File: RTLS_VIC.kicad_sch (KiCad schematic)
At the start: 32 parts, among them J8 Conn_01x02_Pin, SW1 TS-1187A-B-A-B, U2 TPS63900DSKR, U9 STM32F411RET6, X1 XL2EL89COI-111YLC-26M

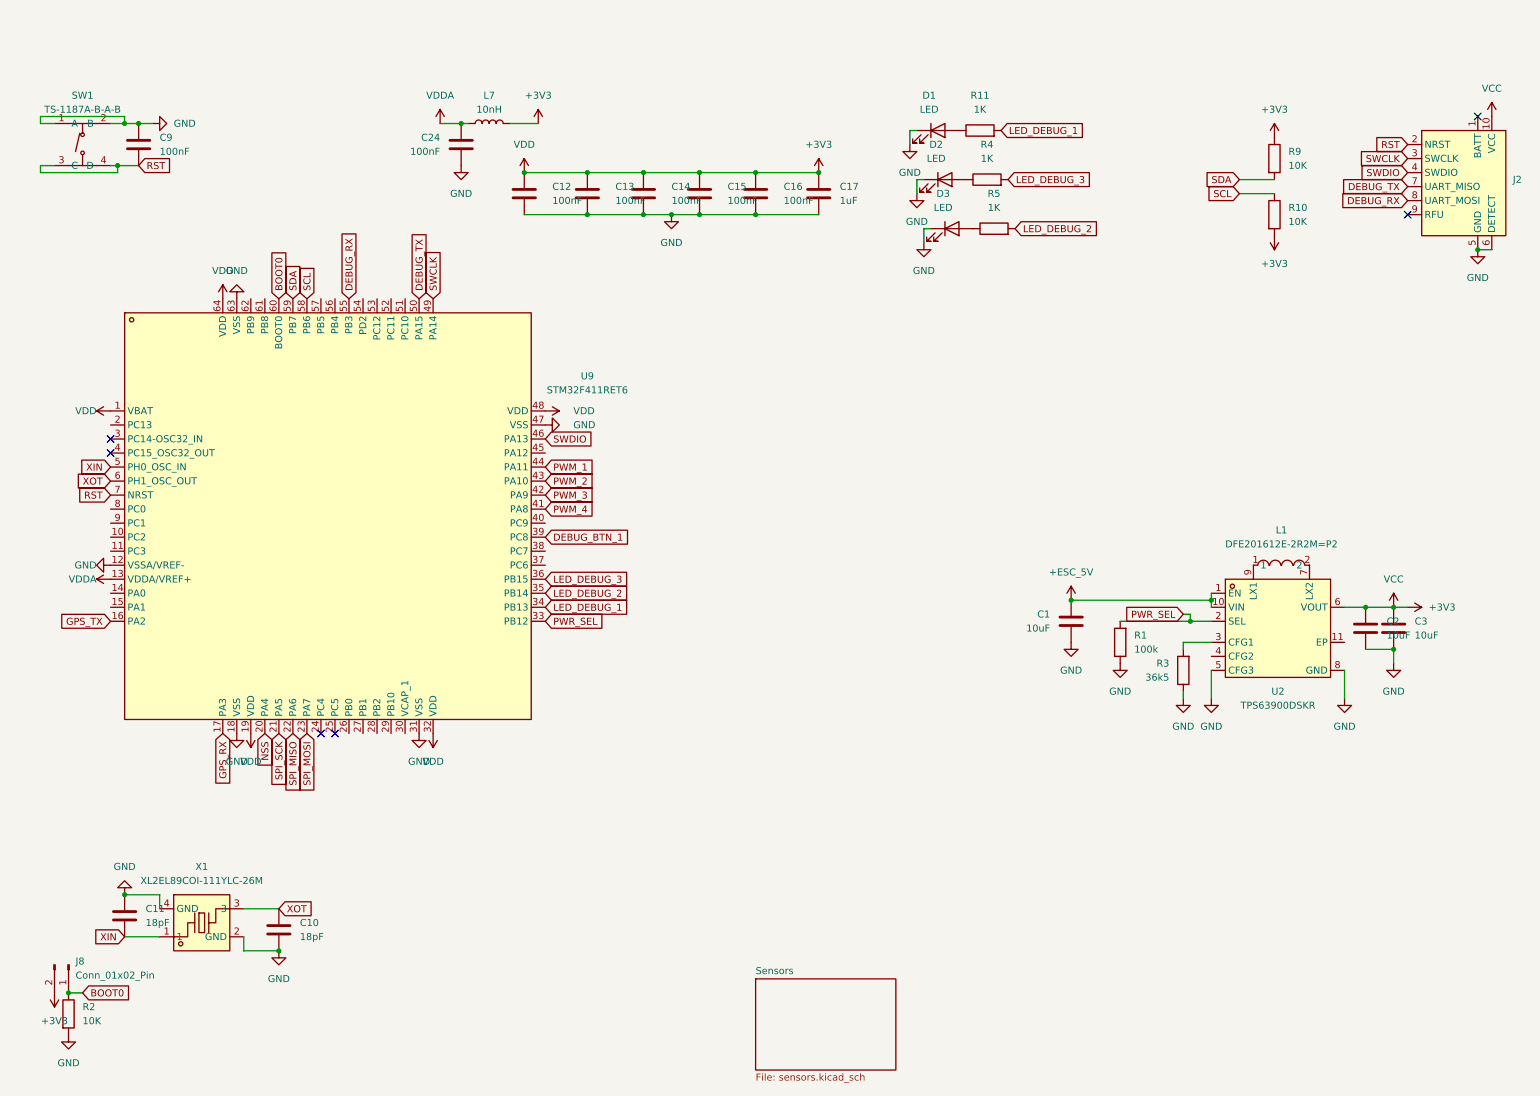
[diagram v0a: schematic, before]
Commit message: nearly there
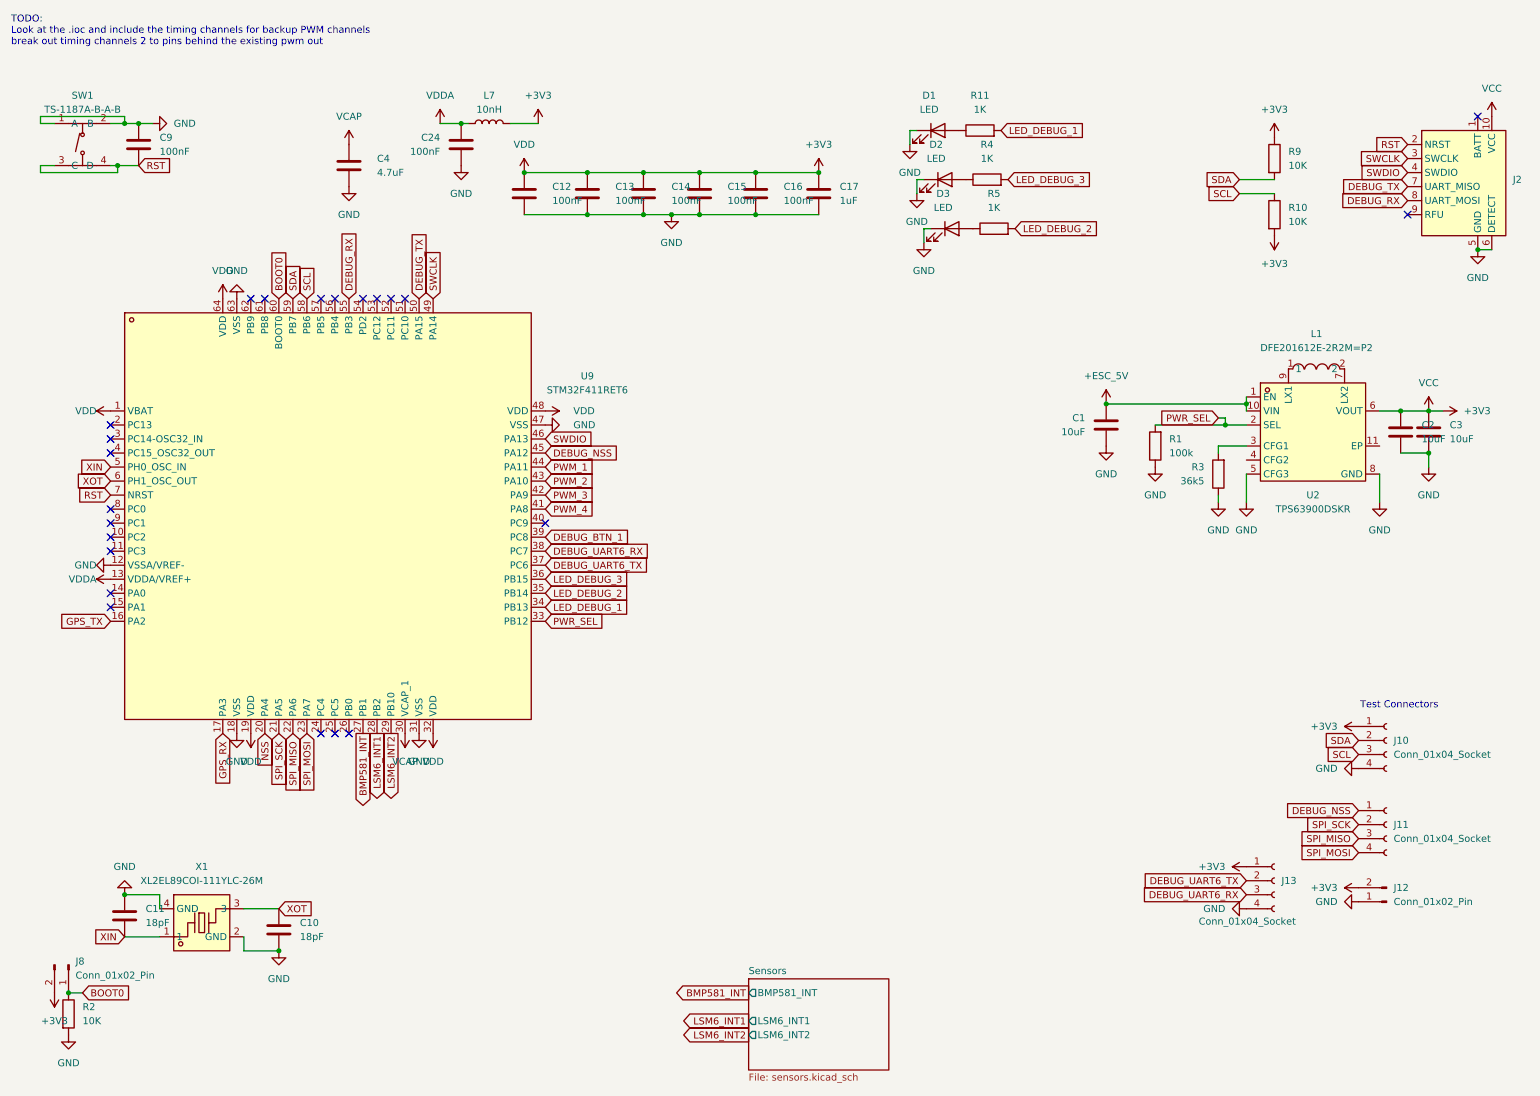
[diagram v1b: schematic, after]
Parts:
- added C4: 4.7uF, Capacitor_SMD:C_0402_1005Metric, symbol Device:C
- added J10, J11, J13: Conn_01x04_Socket, Connector_PinSocket_2.54mm:PinSocket_1x04_P2.54mm_Vertical, symbol Connector:Conn_01x04_Socket
- added J12: Conn_01x02_Pin, Connector_PinHeader_2.54mm:PinHeader_1x02_P2.54mm_Vertical, symbol Connector:Conn_01x02_Pin
- J8: now left out of the parts list
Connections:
- net +3V3: now also J10.1 (Pin_1), J12.2 (Pin_2), J13.1 (Pin_1)
- net GND: now also C4.2, J10.4 (Pin_4), J12.1 (Pin_1), J13.4 (Pin_4)
- net SCL: now also J10.3 (Pin_3)
- net SDA: now also J10.2 (Pin_2)
- net SPI_MISO: now also J11.3 (Pin_3)
- net SPI_MOSI: now also J11.4 (Pin_4)
- net SPI_SCK: now also J11.2 (Pin_2)
- net BMP581_INT: now reaches U9.27 (PB1)
- net LSM6_INT1: now reaches U9.28 (PB2)
- net LSM6_INT2: now reaches U9.29 (PB10)
- net VCAP: now reaches U9.30 (VCAP_1)
- net VCAP: now also C4.1
- net DEBUG_UART6_TX: now reaches U9.37 (PC6)
- net DEBUG_UART6_TX: now also J13.2 (Pin_2)
- net DEBUG_UART6_RX: now reaches U9.38 (PC7)
- net DEBUG_UART6_RX: now also J13.3 (Pin_3)
- net DEBUG_NSS: now reaches U9.45 (PA12)
- net DEBUG_NSS: now also J11.1 (Pin_1)
- no-connect marks 6 -> 23
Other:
- sheet Sensors ports: added BMP581_INT, LSM6_INT1, LSM6_INT2; removed none
- note added: "TODO: Look at the .ioc and include the timing channels for backup PWM channels break out timing channels 2 to pins behind the existing pwm out"
- note added: "Test Connectors"
- moved on the sheet: C1, C2, C3, L1, R1, R3, U2

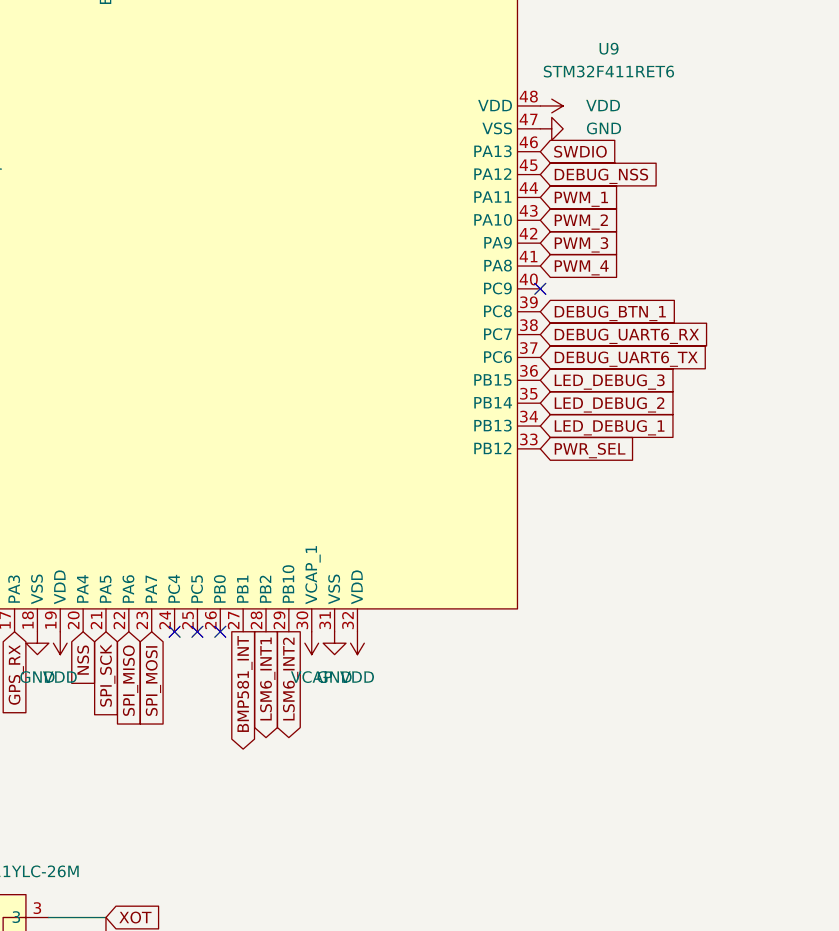
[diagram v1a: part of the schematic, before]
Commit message: preparing for prod
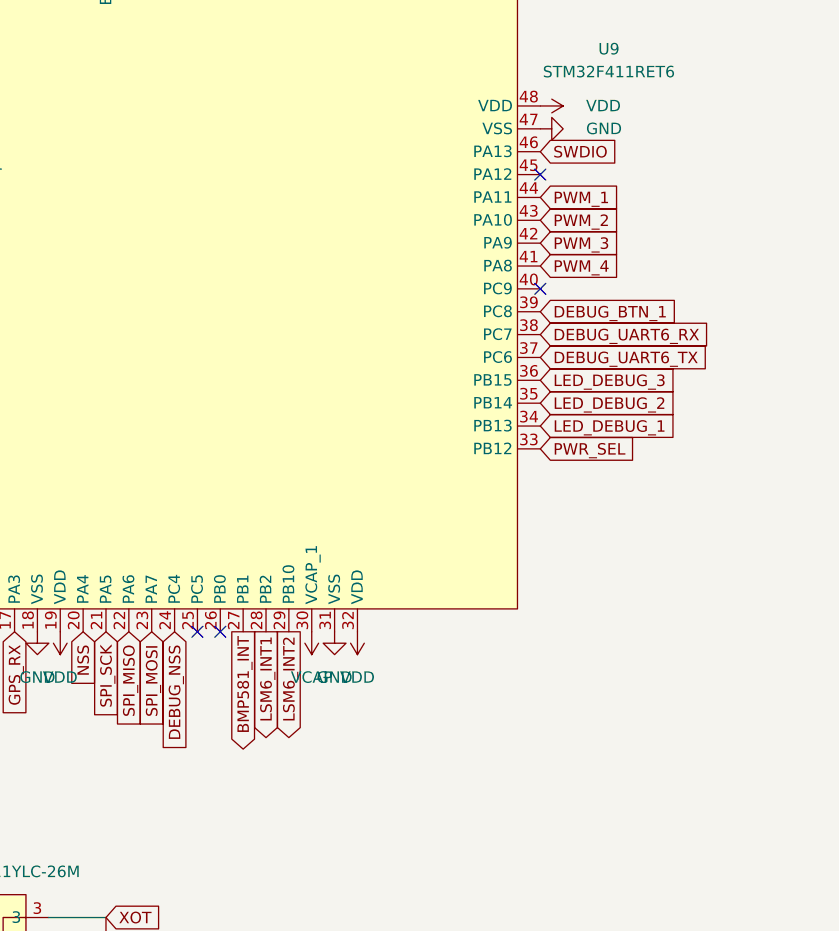
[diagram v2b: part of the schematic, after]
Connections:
- net DEBUG_NSS: now also U9.24 (PC4); no longer U9.45 (PA12)
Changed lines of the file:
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@@
+	)
+	(no_connect
+		(at 106.68 80.01)
 	)
 	(no_connect
@@
 	(no_connect
 		(at 262.89 36.83)
-	)
-	(no_connect
-		(at 66.04 130.81)
 	)
 	(wire
@@
 		)
 	)
+	(global_label "DEBUG_NSS"
+		(shape input)
+		(at 66.04 130.81 270)
+		(fields_autoplaced yes)
+		(effects
+			(font
+				(size 1.27 1.27)
+			)
+			(justify right)
+		)
+		(property "Intersheetrefs" "${INTERSHEET_REFS}"
+			(at 66.04 144.8018 90)
+			(effects
+				(font
+					(size 1.27 1.27)
+				)
+				(justify right)
+				(hide yes)
+			)
+		)
+	)
 	(global_label "LSM6_INT1"
 		(shape output)
@@
 				(hide yes)
 			)
-		)
-	)
-	(global_label "DEBUG_NSS"
-		(shape input)
-		(at 106.68 80.01 0)
-		(fields_autoplaced yes)
-		(effects
-			(font
-				(size 1.27 1.27)
-			)
-			(justify left)
-		)
-		(property "Intersheetrefs" "${INTERSHEET_REFS}"
-			(at 120.6718 80.01 0)
-			(effects
-				(font
-					(size 1.27 1.27)
-				)
-				(justify left)
-				(hide yes)
-			)
